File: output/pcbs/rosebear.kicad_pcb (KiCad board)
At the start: 2 copper layers, 145.1 x 113 mm, 26 parts

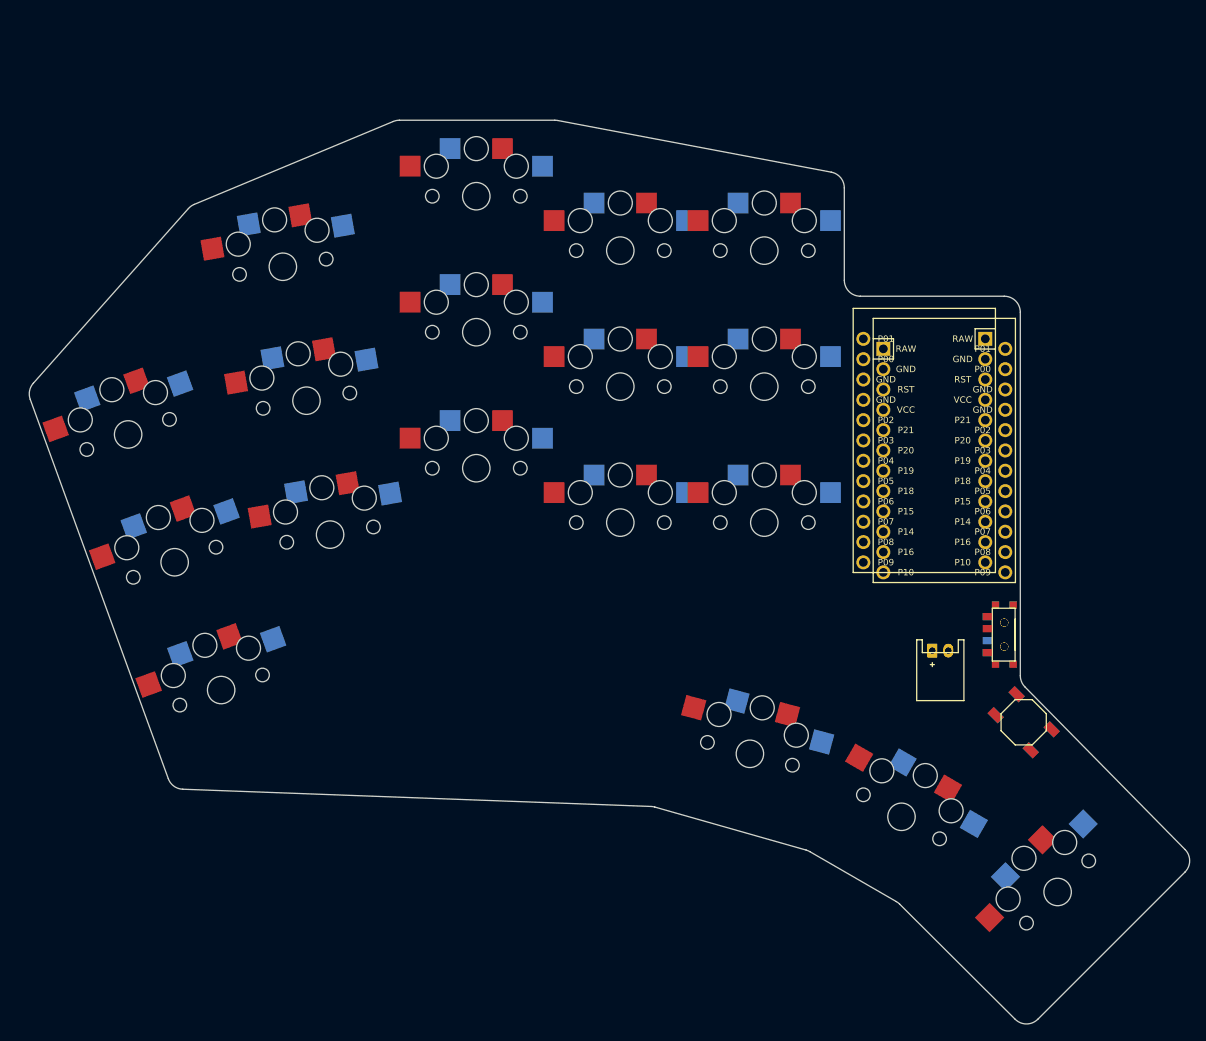
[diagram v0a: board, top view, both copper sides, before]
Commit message: final routing
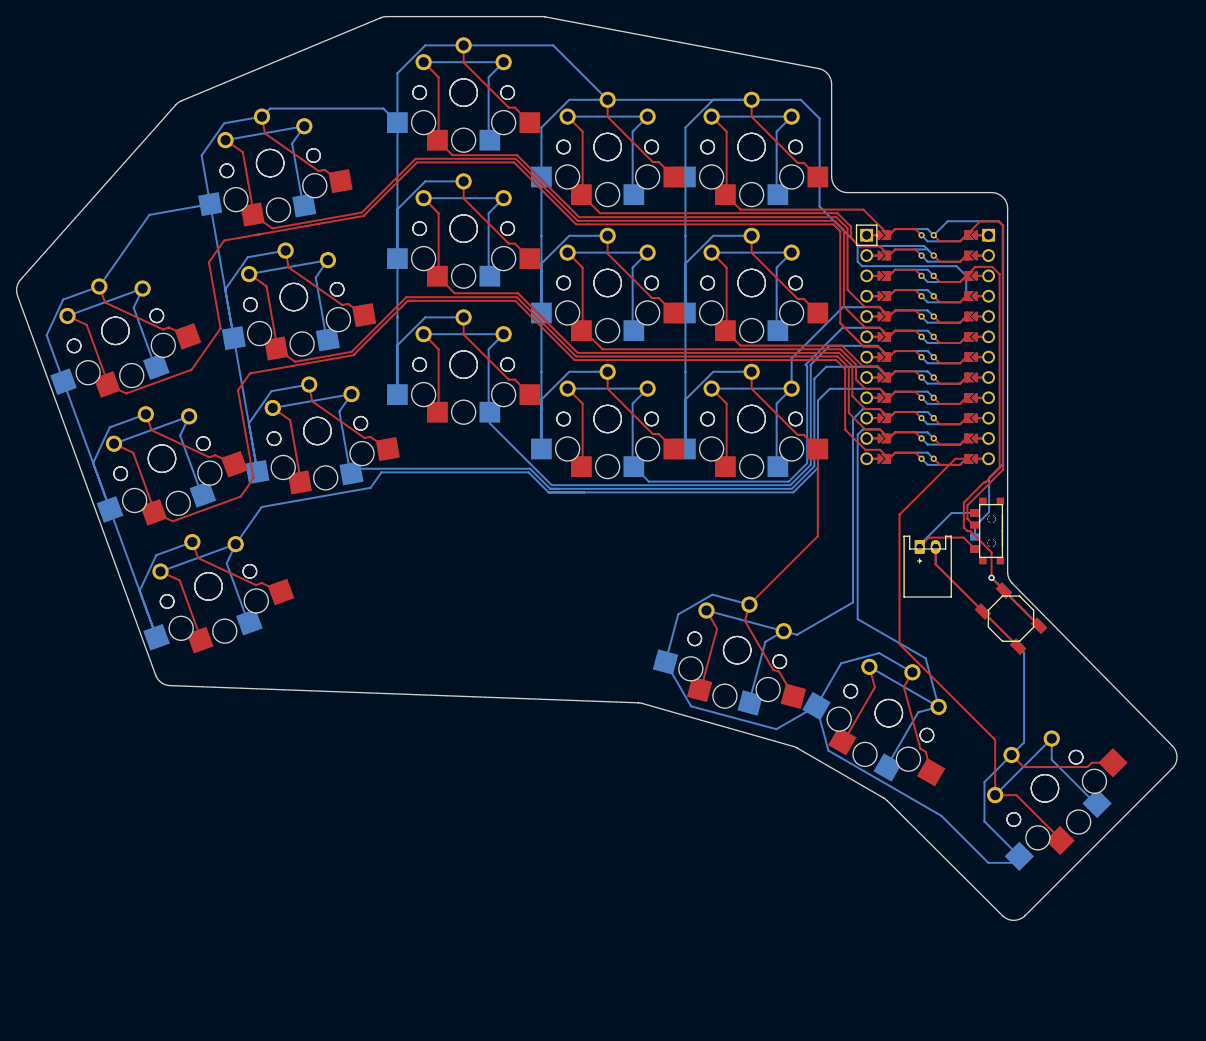
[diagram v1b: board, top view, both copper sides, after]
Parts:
- removed MCU2: , ProMicro
- added S19: , PG1350, F.Cu at (48.4, 87.0)
- added S20: , PG1350, F.Cu at (42.6, 71.1)
- added S21: , PG1350, F.Cu at (36.8, 55.1)
- added S22: , PG1350, F.Cu at (62.0, 67.6)
- added S23: , PG1350, F.Cu at (59.1, 50.9)
- added S24: , PG1350, F.Cu at (56.1, 34.1)
- added S25: , PG1350, F.Cu at (80.3, 59.3)
- added S26: , PG1350, F.Cu at (80.3, 42.3)
- added S27: , PG1350, F.Cu at (80.3, 25.3)
- added S28: , PG1350, F.Cu at (98.3, 66.1)
- added S29: , PG1350, F.Cu at (98.3, 49.1)
- added S30: , PG1350, F.Cu at (98.3, 32.1)
- added S31: , PG1350, F.Cu at (116.3, 66.1)
- added S32: , PG1350, F.Cu at (116.3, 49.1)
- added S33: , PG1350, F.Cu at (116.3, 32.1)
- added S34: , PG1350, F.Cu at (114.5, 95.0)
- added S35: , PG1350, F.Cu at (133.5, 102.9)
- added S36: , PG1350, F.Cu at (153.0, 112.3)
- moved S14 13.0 mm to (116.3, 49.1)
- moved S6 13.0 mm to (56.1, 34.1)
- moved T1 13.0 mm to (146.3, 80.1)
- moved T2 13.0 mm to (146.3, 80.1)
- moved S7 13.0 mm to (80.3, 59.3)
- moved S8 13.0 mm to (80.3, 42.3)
- moved S15 13.0 mm to (116.3, 32.1)
- moved S18 13.0 mm to (153.0, 112.3)
- moved S12 13.0 mm to (98.3, 32.1)
- moved S10 13.0 mm to (98.3, 66.1)
- moved S17 13.0 mm to (133.5, 102.9)
- moved S9 13.0 mm to (80.3, 25.3)
- moved S4 13.0 mm to (62.0, 67.6)
- moved JST1 13.0 mm to (138.3, 82.1)
- moved JST2 13.0 mm to (138.3, 82.1)
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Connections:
- MCU1 pad 13: P1 -> P9
- MCU1 pad 14: P0 -> P8
- MCU1 pad 15: GND -> P7
- MCU1 pad 16: GND -> P6
- MCU1 pad 17: P2 -> P5
- MCU1 pad 18: P3 -> P4
- MCU1 pad 19: P4 -> P3
- MCU1 pad 20: P5 -> P2
- MCU1 pad 21: P6 -> GND
- MCU1 pad 22: P7 -> GND
- MCU1 pad 23: P8 -> P0
- MCU1 pad 24: P9 -> P1
- S1 pad 1: P20 -> P15
- S1 pad 2: pinky_bottom -> GND
- S10 pad 1: P15 -> P20
- S10 pad 2: index_bottom -> GND
- S11 pad 1: P15 -> P6
- S11 pad 2: index_home -> GND
- S12 pad 1: P15 -> P0
- S12 pad 2: index_top -> GND
- S13 pad 1: P14 -> P21
- S13 pad 2: inner_bottom -> GND
- S14 pad 1: P14 -> P5
- S14 pad 2: inner_home -> GND
- S15 pad 1: P14 -> P1
- S15 pad 2: inner_top -> GND
- S16 pad 1: P18 -> P14
- S16 pad 2: near_thumb -> GND
- S17 pad 1: P15 -> P16
- S17 pad 2: home_thumb -> GND
- S18 pad 1: P14 -> P10
- S18 pad 2: far_thumb -> GND
- S2 pad 1: P20 -> P9
- S2 pad 2: pinky_home -> GND
- S3 pad 1: P20 -> P4
- S3 pad 2: pinky_top -> GND
- S4 pad 1: P19 -> P18
- S4 pad 2: ring_bottom -> GND
- S5 pad 1: P19 -> P8
- S5 pad 2: ring_home -> GND
- S6 pad 1: P19 -> P3
- S6 pad 2: ring_top -> GND
- S7 pad 1: P18 -> P19
- S7 pad 2: middle_bottom -> GND
- S8 pad 1: P18 -> P7
- S8 pad 2: middle_home -> GND
- S9 pad 1: P18 -> P2
- S9 pad 2: middle_top -> GND
- T1 pad 1: RAW -> Bplus
- T1 pad 2: Bplus -> RAW
- T2 pad 1: RAW -> Bplus
- T2 pad 2: Bplus -> RAW
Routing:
- net GND: track 0.00 -> 960.7 mm
- net P4: track 0.00 -> 164.3 mm
- net P9: track 0.00 -> 155.9 mm
- net P15: track 0.00 -> 132.7 mm
- net P3: track 0.00 -> 129.1 mm
- net P8: track 0.00 -> 121.9 mm
- net P18: track 0.00 -> 114.0 mm
- net P2: track 0.00 -> 101.3 mm
- net P19: track 0.00 -> 100.8 mm
- net P7: track 0.00 -> 97.2 mm
- net RAW: track 0.00 -> 95.3 mm
- net P10: track 0.00 -> 82.4 mm
- net P20: track 0.00 -> 79.8 mm
- net P16: track 0.00 -> 75.0 mm
- net P6: track 0.00 -> 73.9 mm
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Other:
- net class Default removed
- rule pad_to_mask_clearance: 0.05 -> 0
- board text added: "ROSEBEAR. "
